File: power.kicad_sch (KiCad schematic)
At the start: 29 parts, among them J3 BATTERY, J5 USB_C_Receptacle_USB2.0_16P, SW20 POWER_BUTTON, U4 BQ21040DBV, U6 RT8059

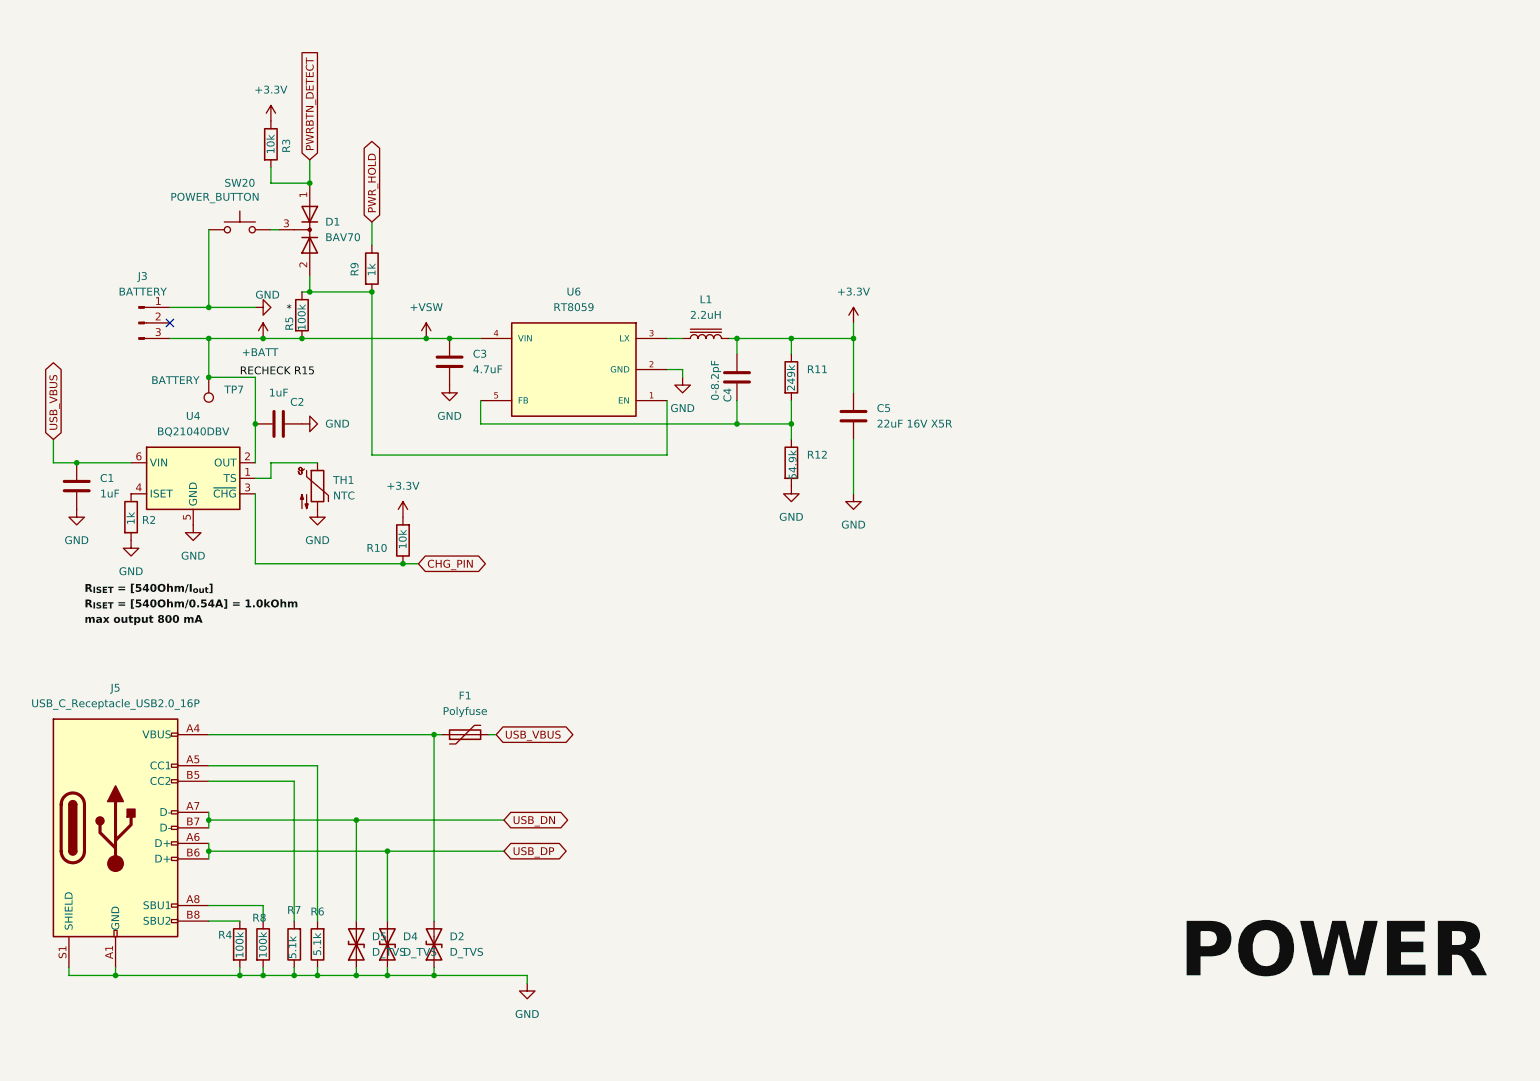
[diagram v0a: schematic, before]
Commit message: SCHEMATIC
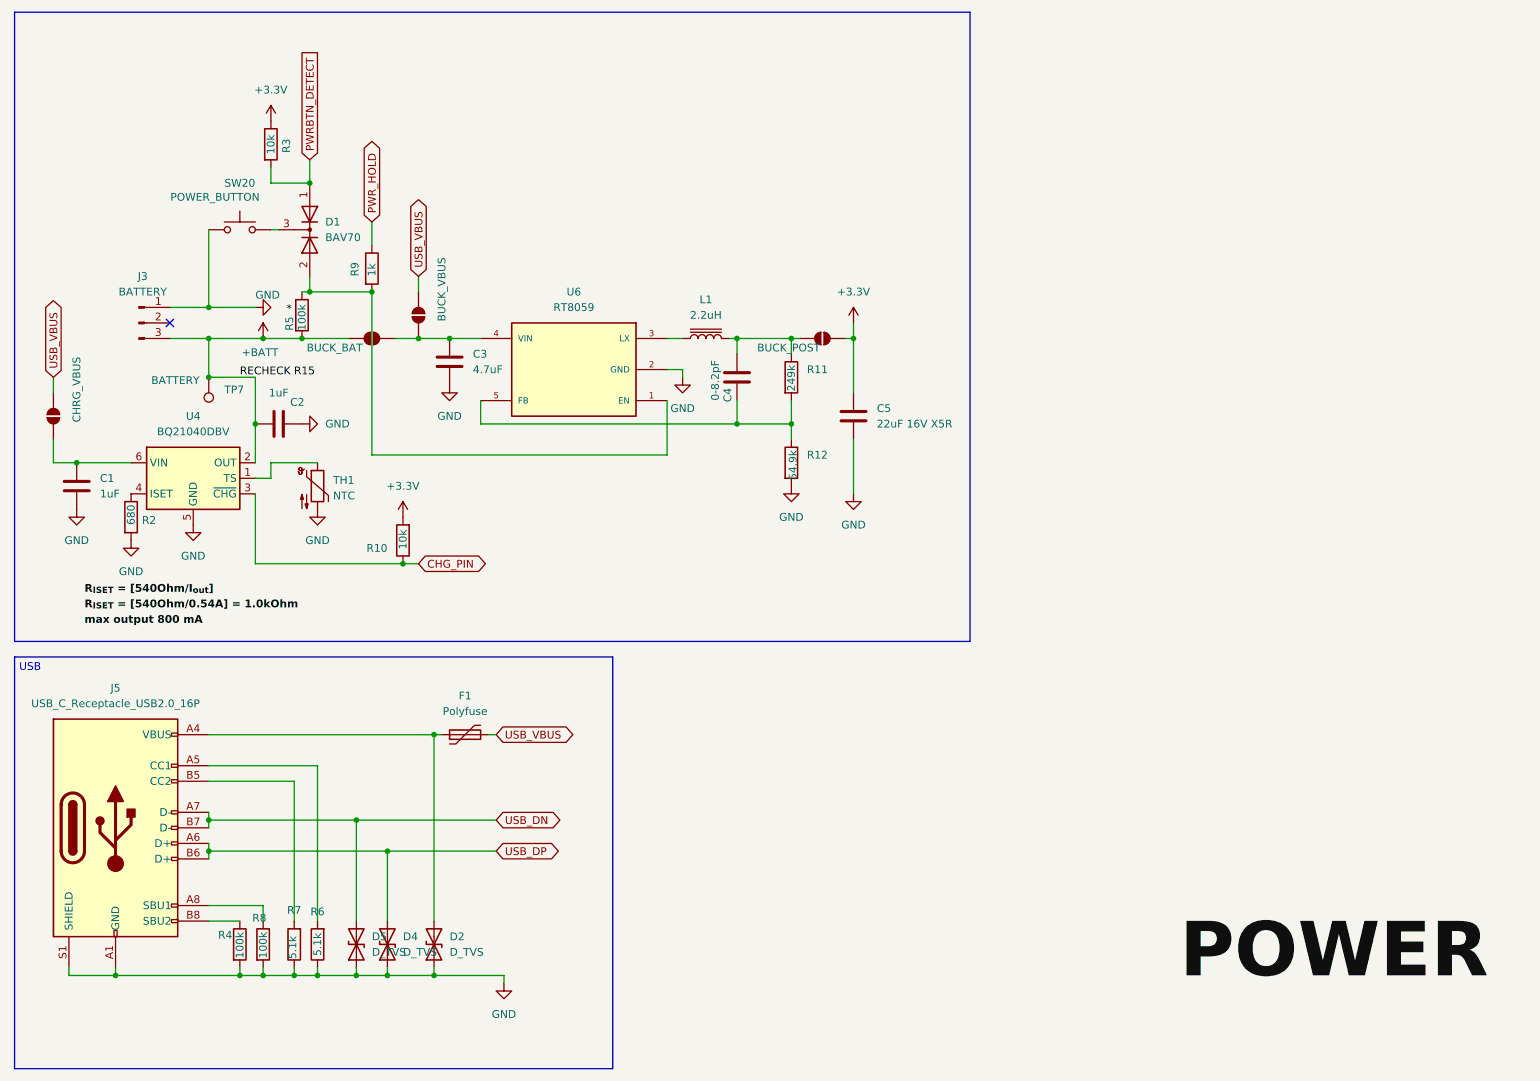
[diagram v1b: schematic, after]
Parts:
- added BUCK_BAT, BUCK_POST, BUCK_VBUS, CHRG_VBUS: SolderJumper_2_Open, Jumper:SolderJumper-2_P1.3mm_Open_Pad1.0x1.5mm, symbol Jumper:SolderJumper_2_Open
- R2: value 1k -> 680
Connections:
- net +3.3V: now also BUCK_POST.1 (A); no longer C4.1, L1.2, R11.1
- net +BATT: now also BUCK_BAT.2 (B); no longer C3.1, U6.4 (VIN)
- net USB_VBUS: now also BUCK_VBUS.1 (A), CHRG_VBUS.1 (A); no longer C1.1, U4.6 (VIN)
- new net: BUCK_POST.2 (B), C4.1, L1.2, R11.1
- new net: BUCK_BAT.1 (A), BUCK_VBUS.2 (B), C3.1, U6.4 (VIN)
- new net: C1.1, CHRG_VBUS.2 (B), U4.6 (VIN)
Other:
- note added: "USB"
